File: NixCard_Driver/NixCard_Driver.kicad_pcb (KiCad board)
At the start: 2 copper layers, 21.6 x 31.8 mm, 13 parts, among them P1 CONN_01X06, P2 CONN_01X06, P3 TSW-104-07-F-S, P4 TSW-104-07-F-S, U1 HV513WG, U2 HV513WG

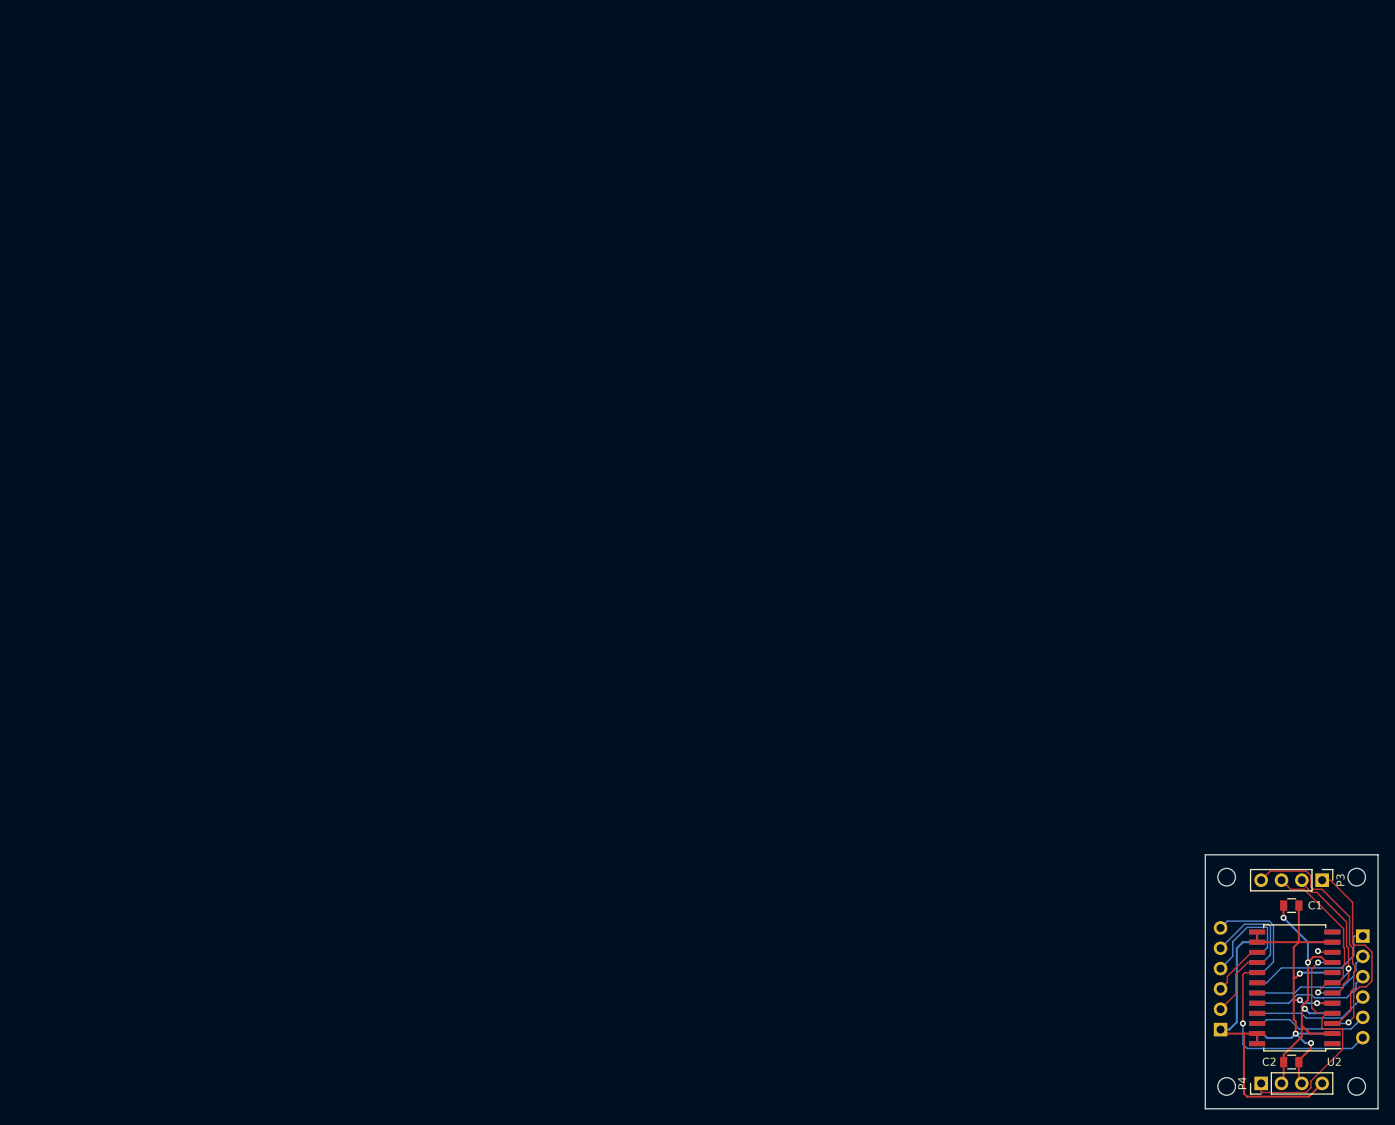
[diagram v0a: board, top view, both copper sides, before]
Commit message: Redo of driver board
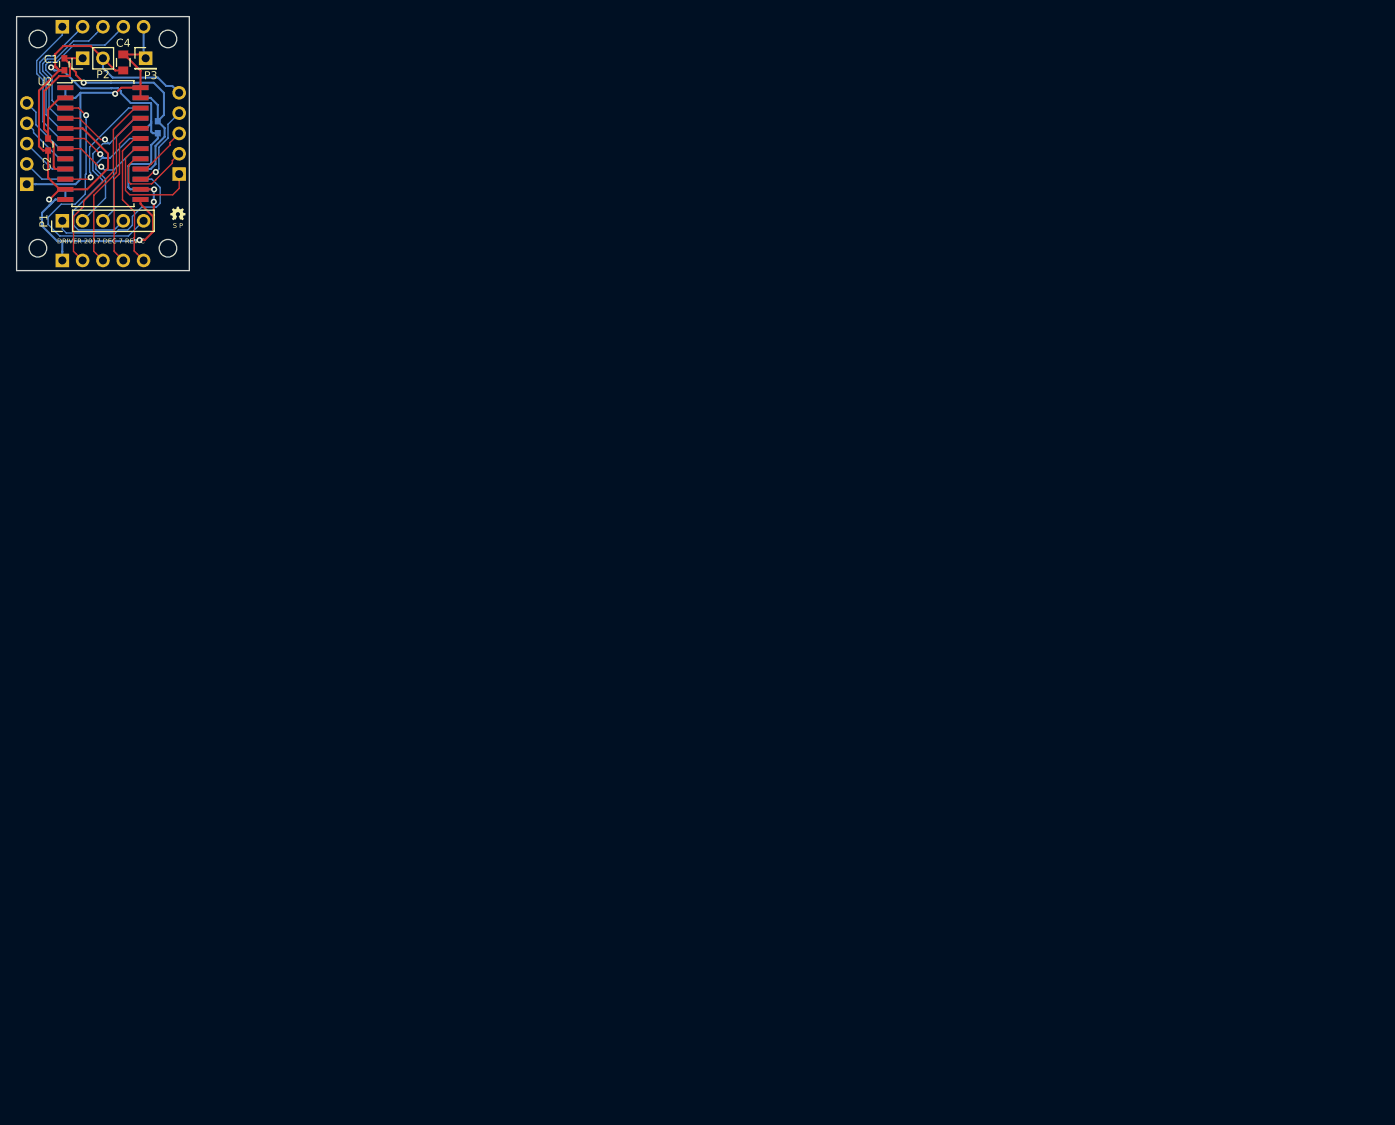
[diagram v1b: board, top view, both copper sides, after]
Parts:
- added C3: 100n, Capacitors_SMD:C_0603, B.Cu at (6.86, -2.04)
- added C4: 100n, Capacitors_SMD:C_0805, F.Cu at (2.54, -10.1)
- added P5: CONN_01X05, Conn_PinHeader_2.54mm:PinHeader_1x05_P2.54mm_Vertical, B.Cu at (-9.53, 5.08)
- added P6: CONN_01X05, Conn_PinHeader_2.54mm:PinHeader_1x05_P2.54mm_Vertical, B.Cu at (-5.08, 14.6)
- added P7: CONN_01X05, Conn_PinHeader_2.54mm:PinHeader_1x05_P2.54mm_Vertical, B.Cu at (9.53, 3.81)
- C1, C2: footprint quad_level_shifter:C_0805 -> Capacitors_SMD:C_0603
- P1: value CONN_01X06 -> CONN_01X05; footprint Pin_Headers:Pin_Header_Straight_1x06_Pitch2.54mm -> Conn_PinHeader_2.54mm:PinHeader_1x05_P2.54mm_Vertical; moved to F.Cu
- P2: value CONN_01X06 -> CONN_01X02; footprint Pin_Headers:Pin_Header_Straight_1x06_Pitch2.54mm -> Conn_PinHeader_2.54mm:PinHeader_1x02_P2.54mm_Vertical; moved to F.Cu
- P3: value TSW-104-07-F-S -> CONN_01X01; footprint Pin_Headers:Pin_Header_Straight_1x04_Pitch2.54mm -> Conn_PinHeader_2.54mm:PinHeader_1x01_P2.54mm_Vertical
- P4: value TSW-104-07-F-S -> CONN_01X05; footprint Pin_Headers:Pin_Header_Straight_1x04_Pitch2.54mm -> Conn_PinHeader_2.54mm:PinHeader_1x05_P2.54mm_Vertical; moved to B.Cu
- svg2mod: moved to F.Cu
- moved P4 199.8 mm to (-5.08, -14.6), turned to 270 degrees
- moved C2 193.2 mm to (-6.86, 0.12), turned to 270 degrees
- moved P2 187.0 mm to (-2.54, -10.7), turned to 90 degrees
- moved C1 186.0 mm to (-4.83, -9.92), turned to 270 degrees
- moved P1 185.5 mm to (-5.08, 9.65), turned to 90 degrees
- moved U1 182.6 mm to (-0.00, 0.00)
- moved U2 182.6 mm to (-0.00, 0.00), turned to 0 degrees
- moved REF** 181.8 mm to (8.13, 13.1)
- moved REF** 181.8 mm to (8.13, -13.1)
- moved REF** 181.8 mm to (-8.13, -13.1)
- moved REF** 181.8 mm to (-8.13, 13.1)
- moved svg2mod 179.8 mm to (9.37, 8.74), turned to 0 degrees
- moved P3 179.4 mm to (5.33, -10.7), turned to 0 degrees
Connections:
- P1 pad 1: /NIX5 -> /DIN
- P1 pad 2: /NIX4 -> /CLK
- P1 pad 3: /NIX3 -> /~LE
- P1 pad 4: /NIX2 -> /~OE
- P1 pad 5: /NIX1 -> /DOUT
- P2 pad 1: VAA -> +5V
- P2 pad 2: /NIX0 -> GNDREF
- P3 pad 1: /DIN -> VAA
- P4 pad 1: /~OE -> /HV4
- P4 pad 2: +5V -> /HV5
- P4 pad 3: GNDREF -> /HV6
- P4 pad 4: VAA -> /HV7
- U1 pad 15: /NIX1 -> /HV0
- U1 pad 16: /NIX2 -> /HV1
- U1 pad 17: /NIX3 -> /HV2
- U1 pad 18: /NIX4 -> /HV3
- U1 pad 19: /NIX5 -> /HV4
- U1 pad 20: /NIX6 -> /HV5
- U1 pad 21: /NIX7 -> /HV6
- U1 pad 22: /NIX8 -> /HV7
- U2 pad 15: /NIX9 -> /HV8
- U2 pad 16: /NIX0 -> /HV9
- U2 pad 17: /NIXDP -> /HV10
- U2 pad 18: Net-(U2-Pad18) -> /HV11
- U2 pad 19: Net-(U2-Pad19) -> /HV12
- U2 pad 20: Net-(U2-Pad20) -> /HV13
- U2 pad 21: Net-(U2-Pad21) -> /HV14
- U2 pad 22: Net-(U2-Pad22) -> /HV15
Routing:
- net GNDREF: track 56.6 -> 130.0 mm
- net /NIXDP: track 26.3 -> 0.00 mm, vias 1 -> 0
- net /HV15: track 0.00 -> 23.4 mm
- net /HV14: track 0.00 -> 21.1 mm
- net /HV13: track 0.00 -> 18.8 mm
- net /HV7: track 0.00 -> 18.5 mm
- net /HV6: track 0.00 -> 17.8 mm
- net /HV12: track 0.00 -> 17.7 mm
- net /HV5: track 0.00 -> 17.2 mm
- net /HV4: track 0.00 -> 17.2 mm
- net /NIX5: track 17.0 -> 0.00 mm
- net +5V: track 40.0 -> 56.3 mm, vias 3 -> 1
- net /NIX4: track 15.9 -> 0.00 mm
- net /HV11: track 0.00 -> 15.5 mm
- net /NIX3: track 15.2 -> 0.00 mm
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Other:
- board text added: "DRIVER 2017 DEC 7 REV C"
- board text added: "VAA"
- board text removed: "+170V"
- board text removed: "BRD B REV C 2017 DEC 2"
